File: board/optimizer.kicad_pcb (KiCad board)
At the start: 2 copper layers, 100 x 55 mm, 64 parts, among them J1 Telemetry, J2 IN+, J3 IN-, J4 OUT-, J5 OUT+, Q1 AOB2500L, U1 MCP1416, U2 LM317_TO-252, U3 AP1117-33, U4 ATSAMD09C13A-SS, X1 SWD

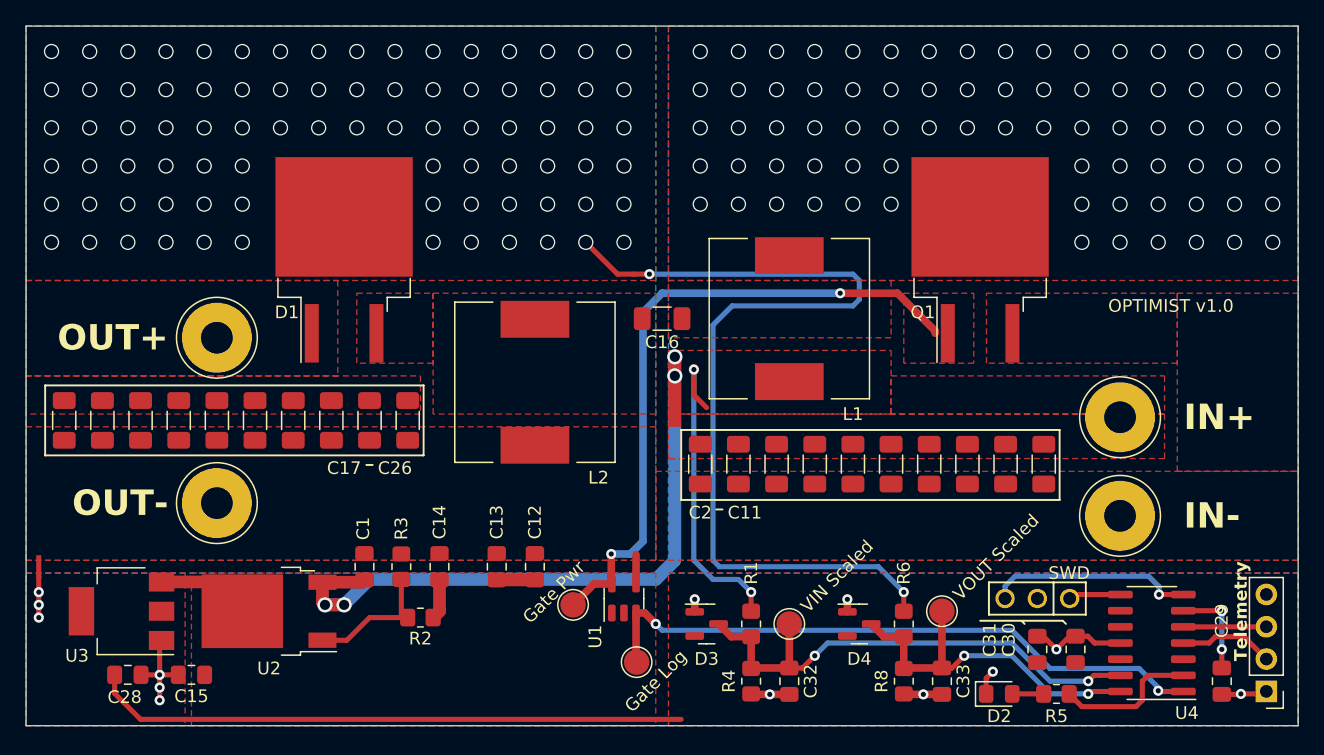
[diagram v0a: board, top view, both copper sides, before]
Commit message: WIP
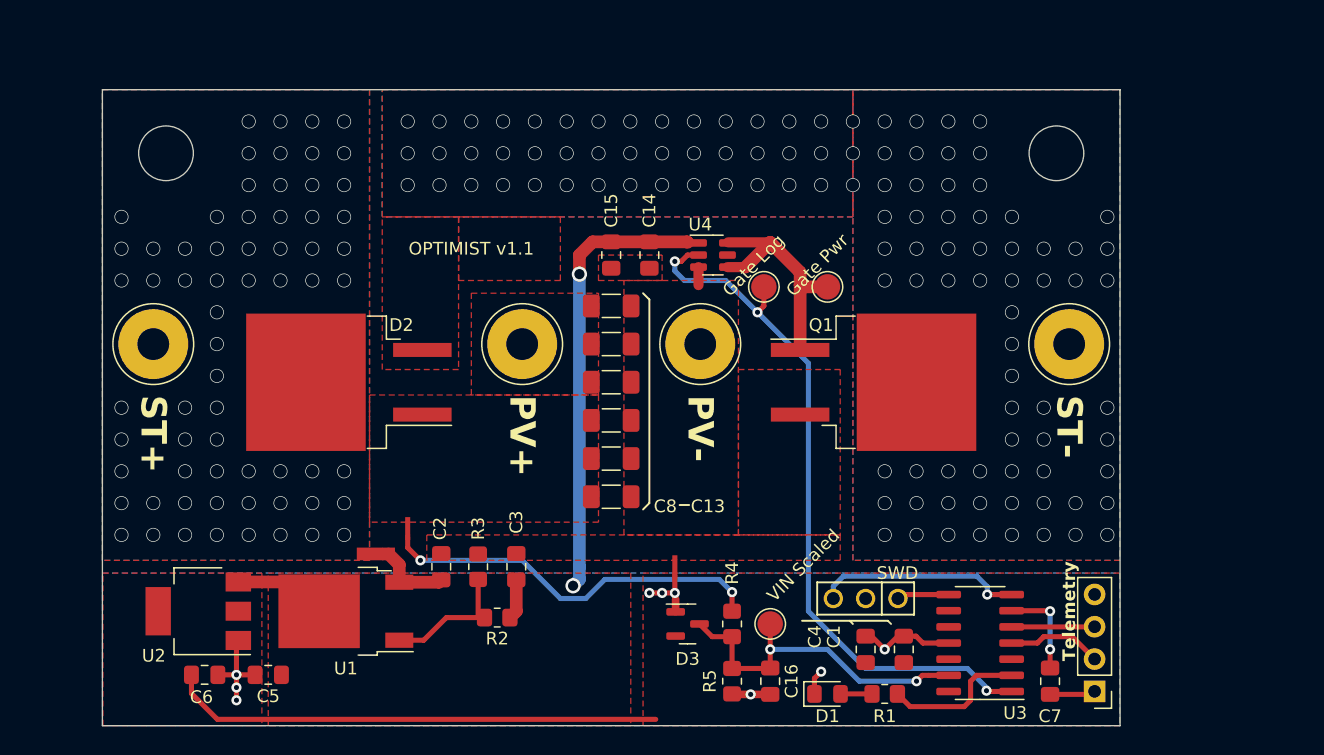
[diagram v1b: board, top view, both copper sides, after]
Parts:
- removed the C10 at (166.0, 124.4)
- removed the C11 at (163.0, 124.4)
- removed the C16 at (160.0, 113.0)
- removed the C2 at (190.0, 124.4)
- removed C22, C23, C24, C25, C26: 10u/50V, Capacitor_SMD:C_1206_3216Metric_Pad1.33x1.80mm_HandSolder
- removed the C3 at (187.0, 124.4)
- removed C33: 100n, Capacitor_SMD:C_0805_2012Metric_Pad1.18x1.45mm_HandSolder
- removed the C4 at (184.0, 124.4)
- removed the C5 at (181.0, 124.4)
- removed the C6 at (178.0, 124.4)
- removed the C7 at (175.0, 124.4)
- removed the C9 at (169.0, 124.4)
- removed D4: BAT54S, Package_TO_SOT_SMD:SOT-23
- removed L1, L2: 1uH/14A, Inductor_SMD:L_12x12mm_H8mm
- removed NT4: NetTie_2, optimizer:NetTie 0.4 mm
- removed R6: 10k, Resistor_SMD:R_0805_2012Metric_Pad1.20x1.40mm_HandSolder
- removed R8: 270R, Resistor_SMD:R_0805_2012Metric_Pad1.20x1.40mm_HandSolder
- removed TP4: VOUT Scaled, TestPoint:TestPoint_Pad_D2.0mm
- removed the U1 at (157.0, 135.0)
- added H1: MountingHole, MountingHole:MountingHole_4.3mm_M4_ISO7380, F.Cu at (121.0, 100.0)
- added H2: MountingHole, MountingHole:MountingHole_4.3mm_M4_ISO7380, F.Cu at (191.0, 100.0)
- added U4: ZXGD3009E6, Package_TO_SOT_SMD:SOT-23-6, F.Cu at (164.0, 108.0)
- J1: renamed from J2; value IN+ -> PV+
- J2: renamed from J5; value OUT+ -> ST+
- J3: value IN- -> PV-
- J4: value OUT- -> ST-
- moved J4 68.2 mm to (192.0, 115.0), turned to 180 degrees
- moved NT3 50.0 mm to (161.0, 132.5)
- moved J1 47.4 mm to (149.0, 115.0)
- moved J3 35.7 mm to (163.0, 115.0), turned to 180 degrees
- moved TP2 32.0 mm to (173.0, 110.5)
- moved TP1 31.1 mm to (168.0, 110.5)
- moved C13 28.6 mm to (156.0, 127.0), turned to 180 degrees
- moved NT1 26.2 mm to (137.5, 131.5), turned to 0 degrees
- moved C14 26.1 mm to (159.0, 108.0), turned to -90 degrees
- moved C15 26.1 mm to (156.0, 108.0), turned to -90 degrees
- moved NT2 25.5 mm to (140.0, 129.5), turned to -90 degrees
- moved C12 25.2 mm to (156.0, 124.0), turned to 180 degrees
- moved C11 22.0 mm to (156.0, 121.0), turned to 180 degrees
- moved C8 20.3 mm to (156.0, 112.0), turned to 180 degrees
- moved C10 19.2 mm to (156.0, 118.0), turned to 180 degrees
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- renumbered C30 to C1, C18 to C10, C19 to C11, C20 to C12, C21 to C13, C12 to C14, C13 to C15, C32 to C16, C1 to C2, C14 to C3, C31 to C4, C15 to C5, C28 to C6, C29 to C7, C17 to C9, D2 to D1, D1 to D2, J1 to J5, NT3 to NT2, NT2 to NT3, R5 to R1, R1 to R4, R4 to R5, TP3 to TP2, TP2 to TP3, U2 to U1, U3 to U2, U4 to U3
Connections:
- net /GATE renamed /GATE_LOG
- net /SWITCH_PATH2 renamed /GATE_PWR
- net /V_IN_FULL renamed /V_FULL
- net /V_IN_SCALE renamed /V_SCALE
- C10 pad 2: /PWR_OUT -> /PWR_P
- C11 pad 2: /PWR_OUT -> /PWR_P
- C12 pad 2: /PWR_OUT -> /PWR_P
- C13 pad 2: /PWR_OUT -> /PWR_P
- C8 pad 2: /PWR_IN -> /PWR_P
- C9 pad 2: /PWR_OUT -> /PWR_P
- D2 pad 1: /PWR_OUT -> /PWR_P
- D2 pad 2: /PWR_PATH2 -> /PWR_GND_OUT
- J1 pad 1: /PWR_IN -> /PWR_P
- J2 pad 1: /PWR_OUT -> /PWR_P
- J4 pad 1: /PWR_GND -> /PWR_GND_OUT
- NT1 pad 1: /PWR_IN -> /PWR_P
- NT2 pad 1: /PWR_IN -> /PWR_P
- Q1 pad 2: /PWR_PATH1 -> /PWR_GND_OUT
- U3 pad 14: /V_OUT_SCALE -> unconnected-(U3-PA04)
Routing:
- net /V_OUT_FULL: track 66.6 -> 0.00 mm, vias 2 -> 0
- net /SWITCH_PATH1: track 54.7 -> 5.94 mm, vias 4 -> 0
- net /GATE_PWR: track 52.0 -> 19.1 mm, vias 2 -> 0
- net +12V: track 13.5 -> 45.6 mm, vias 0 -> 2
- net /V_OUT_SCALE: track 28.7 -> 0.00 mm, vias 2 -> 0
- net /V_SCALE: track 40.2 -> 27.2 mm
- net /V_FULL: track 22.2 -> 30.5 mm
- net +3V3: track 46.8 -> 38.8 mm
- net /GATE_LOG: track 49.6 -> 56.8 mm, vias 2 -> 3
- net /PWR_OUT: track 4.84 -> 0.00 mm, vias 84 -> 0
- net GND: track 32.2 -> 28.7 mm, vias 13 -> 9
- net /PWR_IN: track 2.21 -> 0.00 mm
- net /PWR_GND: track 2.31 -> 1.41 mm
- net /PWR_PATH1: vias 78 -> 0
- net /PWR_P: vias 0 -> 66
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- added copper zone on B.Cu, net /PWR_GND_OUT
- added copper zone on F.Cu, net /PWR_GND_OUT
- added copper zone on B.Cu, net /PWR_P
- added copper zone on F.Cu, net /PWR_P
- removed copper zone on F.Cu, net /GATE_PWR
- removed copper zone on F.Cu, net /PWR_IN
- removed copper zone on B.Cu, net /PWR_OUT
- removed copper zone on F.Cu, net /PWR_OUT
- removed copper zone on B.Cu, net /PWR_PATH1
- removed copper zone on F.Cu, net /PWR_PATH1
- removed copper zone on F.Cu, net /PWR_PATH2
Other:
- board size 100 x 55 mm -> 80 x 50 mm
- board text added: "Address"
- board text added: "OPTIMIST v1.1"
- board text removed: "OPTIMIST v1.0"
